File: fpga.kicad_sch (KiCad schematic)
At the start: 10 parts, among them U10 P0082_BOTTOMMOUNT, Y1 XLL735080.000000I

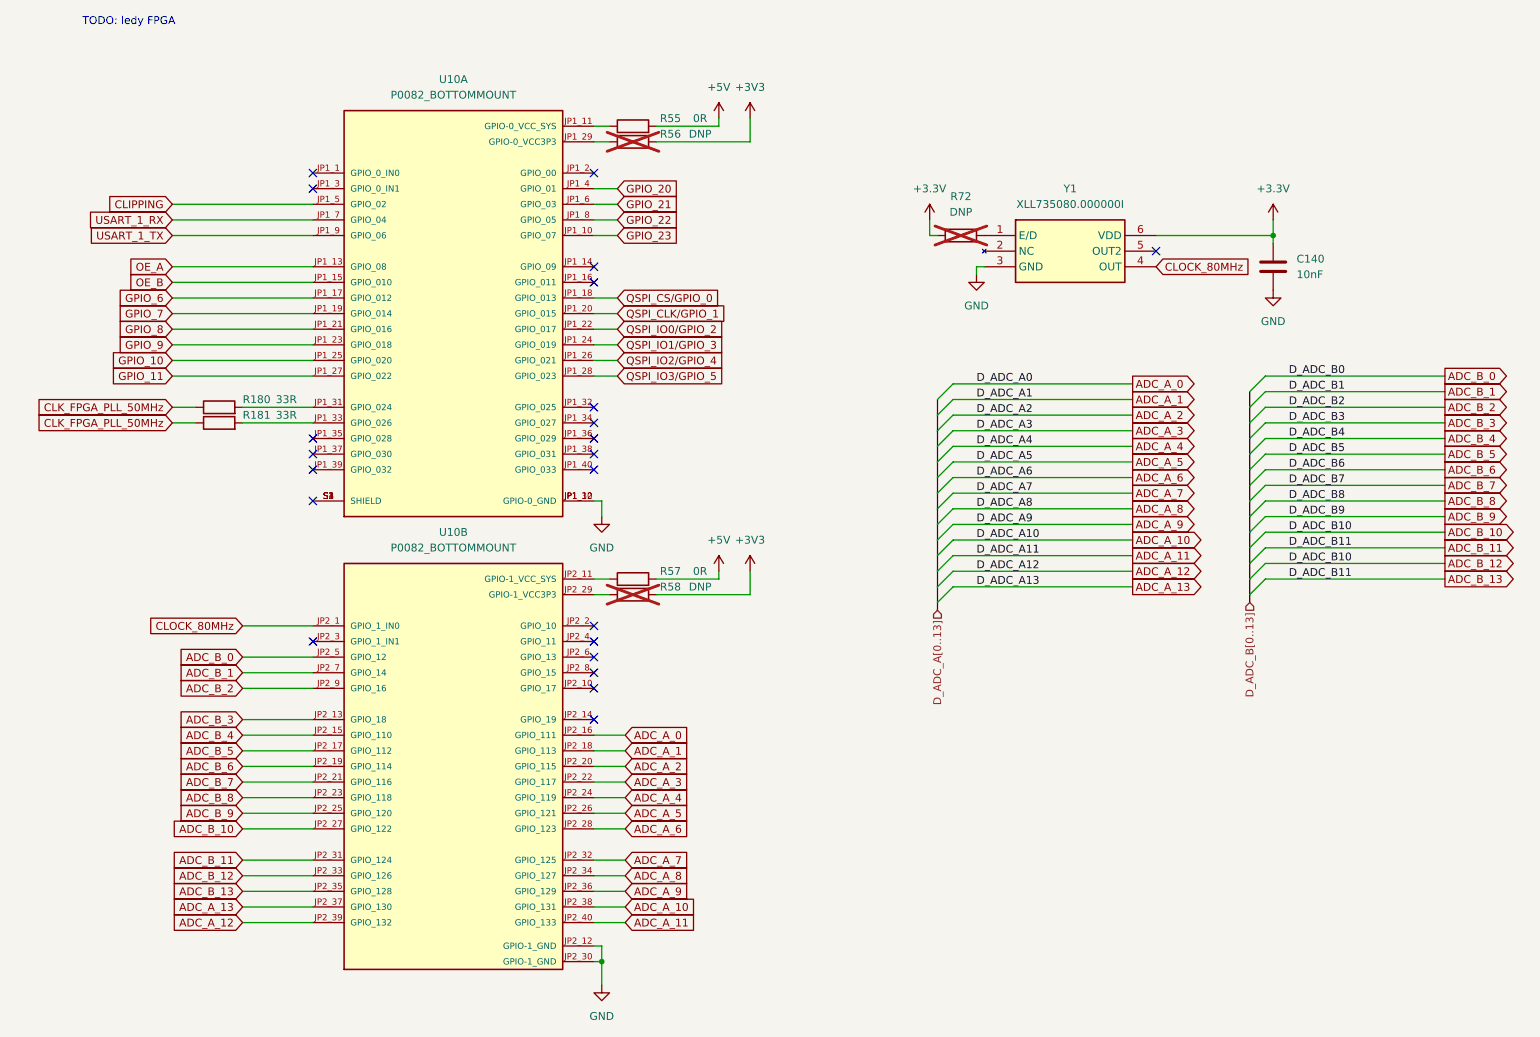
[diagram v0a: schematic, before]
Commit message: Fix ERC
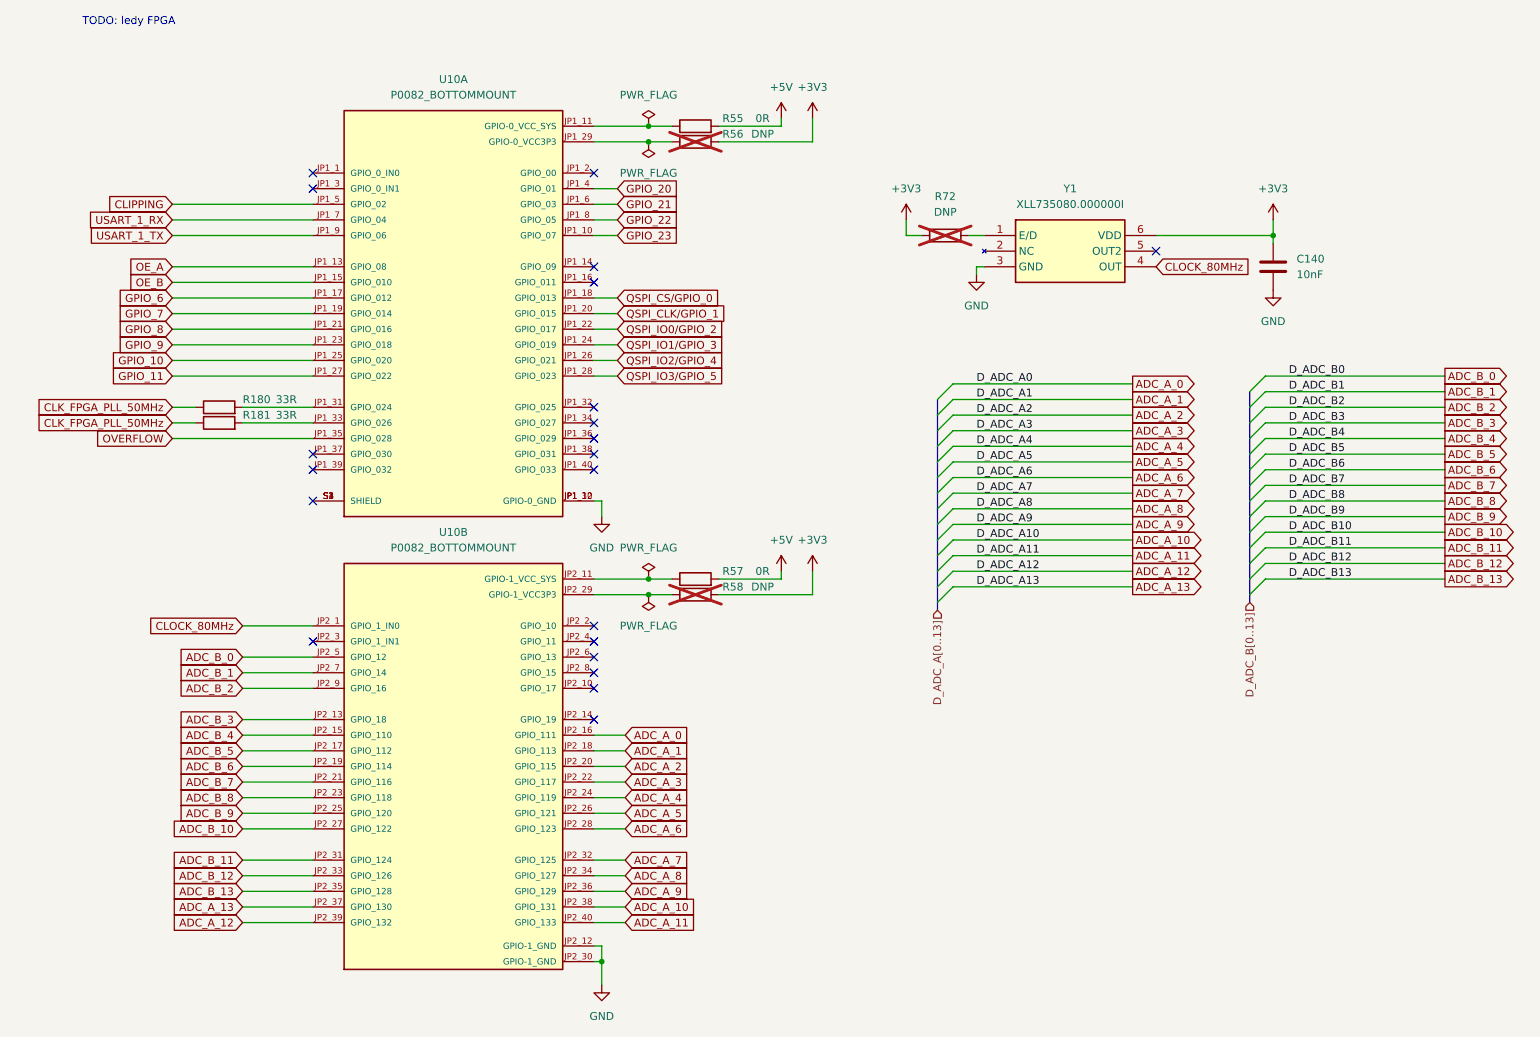
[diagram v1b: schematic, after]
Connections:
- net +3.3V is gone; now on net +3V3: C140.1, R72.1, Y1.6 (VDD)
- net ADC_B_10: no longer U10.JP2_33 (GPIO_126)
- net ADC_B_11: no longer U10.JP2_35 (GPIO_128)
- net OVERFLOW: now reaches U10.JP1_35 (GPIO_028)
- new net ADC_B_12: U10.JP2_33 (GPIO_126)
- new net ADC_B_13: U10.JP2_35 (GPIO_128)
- no-connect marks 22 -> 21
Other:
- moved on the sheet: R55, R56, R57, R58, R72
